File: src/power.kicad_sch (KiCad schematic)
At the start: 28 parts, among them U1 ECP5U_12_CABGA256, U12 TLV62569DRL, U13 TLV62569DRL, U14 TLV62569DRL

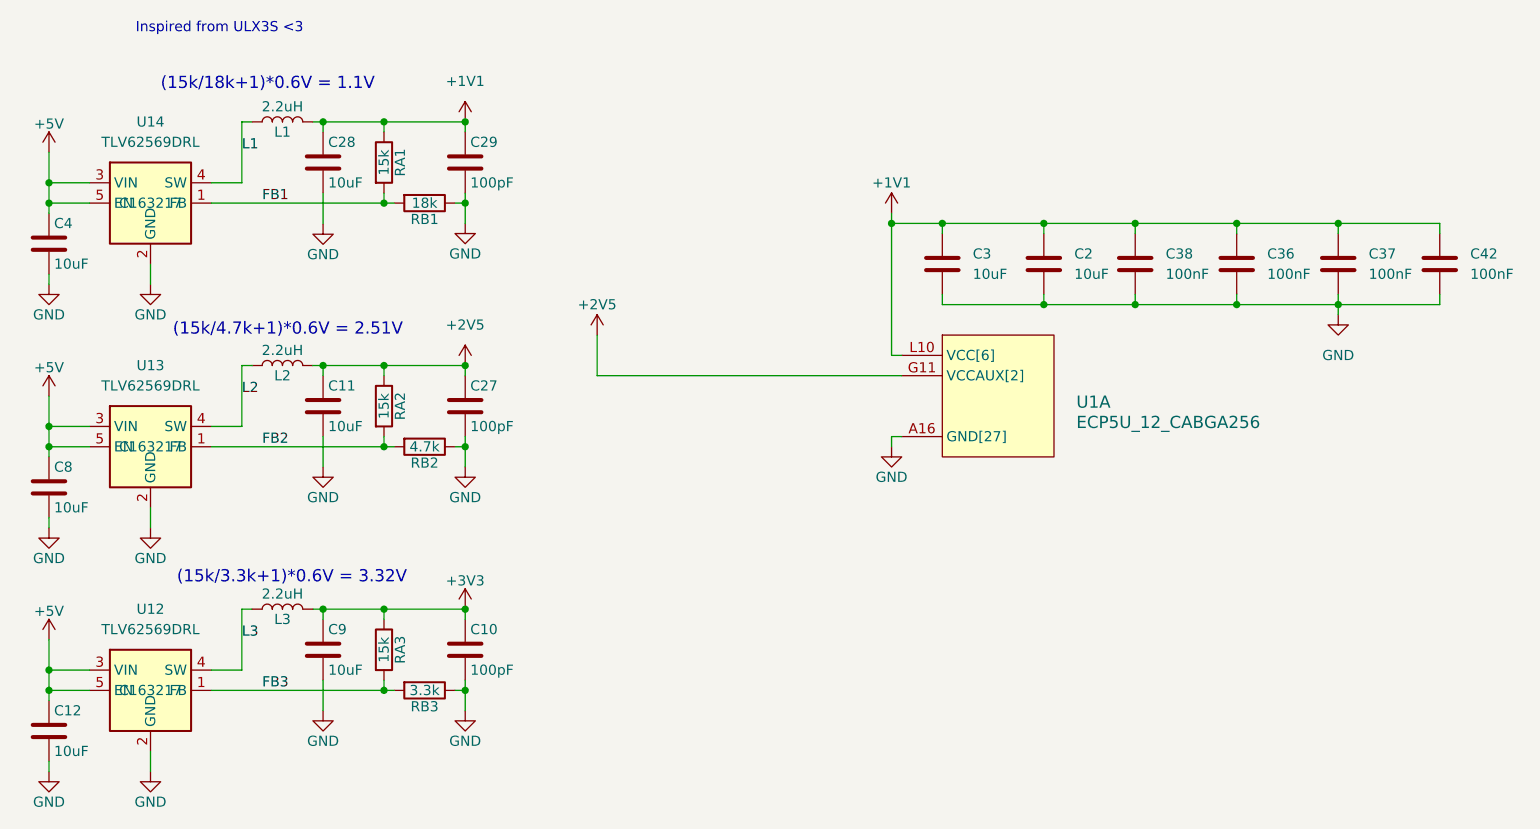
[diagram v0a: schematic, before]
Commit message: Rev 2
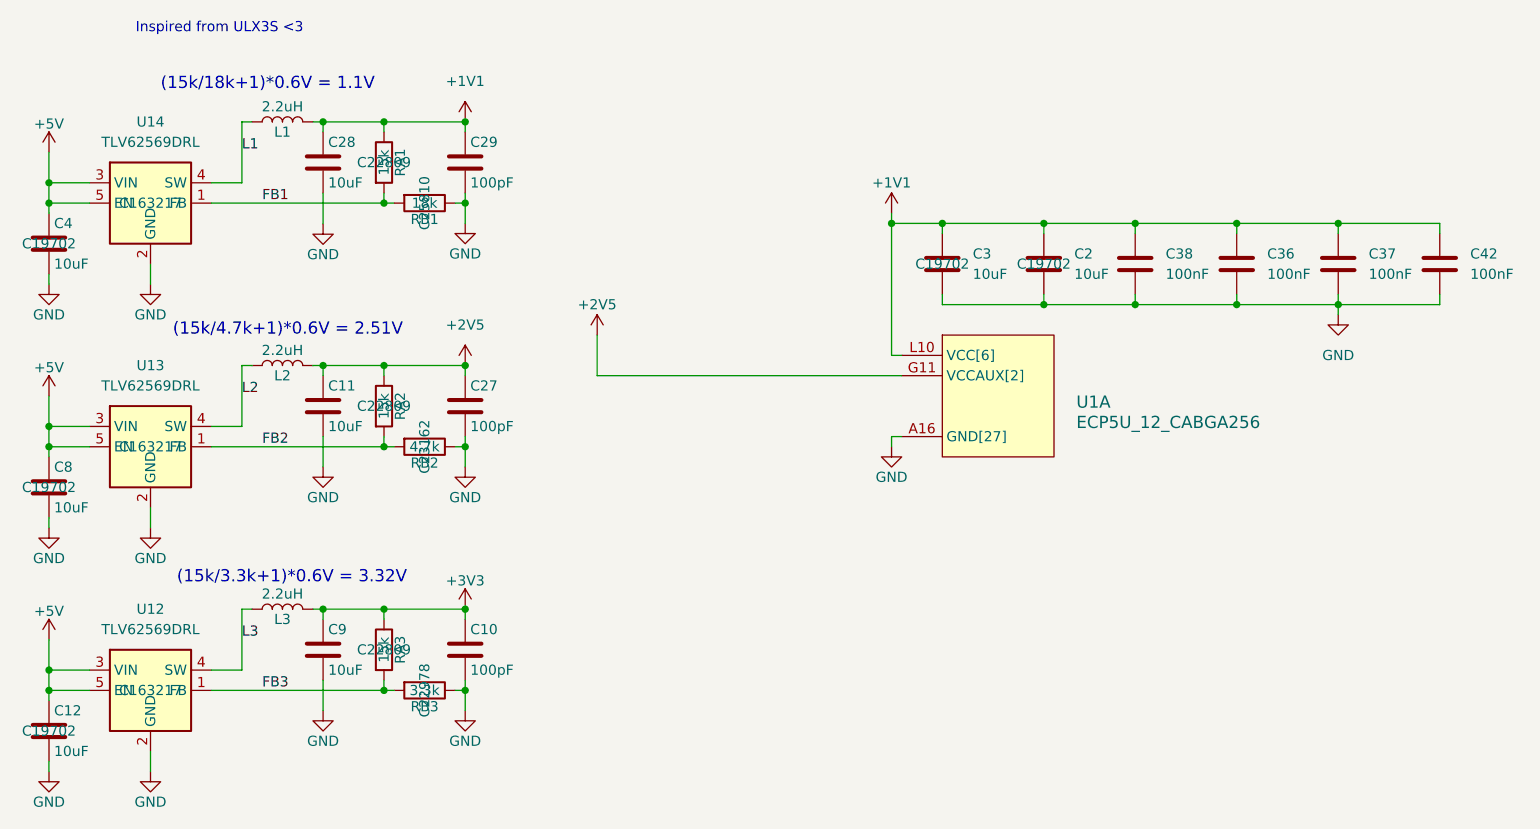
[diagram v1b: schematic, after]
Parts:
- C10, C27, C29: LCSC Part (none) -> C14858
- C11, C12, C2, C28, C3, C4, C8, C9: LCSC Part (none) -> C19702
- C36, C37, C38, C42: LCSC Part (none) -> C1525
- RA1, RA2, RA3: LCSC Part (none) -> C22809
- RB1: LCSC Part (none) -> C25810
- RB2: LCSC Part (none) -> C23162
- RB3: LCSC Part (none) -> C22978
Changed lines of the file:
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@@
 			)
 		)
+		(property "LCSC Part" "C19702"
+			(at 72.39 72.39 0)
+			(effects
+				(font
+					(size 1.27 1.27)
+				)
+			)
+		)
 		(pin "1"
 		)
@@
 			)
 		)
+		(property "LCSC Part" "C22809"
+			(at 114.3 62.23 0)
+			(effects
+				(font
+					(size 1.27 1.27)
+				)
+			)
+		)
 		(pin "1"
 		)
@@
 			)
 		)
+		(property "LCSC Part" "C25810"
+			(at 119.38 67.31 0)
+			(effects
+				(font
+					(size 1.27 1.27)
+				)
+			)
+		)
 		(pin "1"
 		)
@@
 			)
 		)
-		(property "LCSC Part" ""
+		(property "LCSC Part" "C19702"
 			(at 106.68 123.19 0)
 			(effects
@@
 			)
 		)
+		(property "LCSC Part" "C22809"
+			(at 114.3 123.19 0)
+			(effects
+				(font
+					(size 1.27 1.27)
+				)
+			)
+		)
 		(pin "1"
 		)
@@
 			)
 		)
+		(property "LCSC Part" "C22978"
+			(at 119.38 128.27 0)
+			(effects
+				(font
+					(size 1.27 1.27)
+				)
+			)
+		)
 		(pin "1"
 		)
@@
 			)
 		)
-		(property "LCSC Part" ""
+		(property "LCSC Part" "C14858"
 			(at 124.46 123.19 0)
 			(effects
@@
 			)
 		)
+		(property "LCSC Part" "C22809"
+			(at 114.3 92.71 0)
+			(effects
+				(font
+					(size 1.27 1.27)
+				)
+			)
+		)
 		(pin "1"
 		)
@@
 			)
 		)
+		(property "LCSC Part" "C23162"
+			(at 119.38 97.79 0)
+			(effects
+				(font
+					(size 1.27 1.27)
+				)
+			)
+		)
 		(pin "1"
 		)
@@
 			)
 		)
-		(property "LCSC Part" ""
+		(property "LCSC Part" "C1525"
 			(at 246.38 74.93 0)
 			(effects
@@
 			)
 		)
-		(property "LCSC Part" ""
+		(property "LCSC Part" "C14858"
 			(at 124.46 92.71 0)
 			(effects
@@
 			)
 		)
+		(property "LCSC Part" "C19702"
+			(at 72.39 133.35 0)
+			(effects
+				(font
+					(size 1.27 1.27)
+				)
+			)
+		)
 		(pin "1"
 		)
@@
 			)
 		)
-		(property "LCSC Part" ""
+		(property "LCSC Part" "C14858"
 			(at 124.46 62.23 0)
 			(effects
@@
 			)
 		)
-		(property "LCSC Part" ""
+		(property "LCSC Part" "C1525"
 			(at 208.28 74.93 0)
 			(effects
@@
 			)
 		)
+		(property "LCSC Part" "C19702"
+			(at 72.39 102.87 0)
+			(effects
+				(font
+					(size 1.27 1.27)
+				)
+			)
+		)
 		(pin "1"
 		)
@@
 			)
 		)
-		(property "LCSC Part" ""
+		(property "LCSC Part" "C1525"
 			(at 233.68 74.93 0)
 			(effects
@@
 			)
 		)
+		(property "LCSC Part" "C19702"
+			(at 196.85 74.93 0)
+			(effects
+				(font
+					(size 1.27 1.27)
+				)
+			)
+		)
 		(pin "2"
 		)
@@
 			)
 		)
-		(property "LCSC Part" ""
+		(property "LCSC Part" "C19702"
 			(at 106.68 92.71 0)
 			(effects
@@
 			)
 		)
-		(property "LCSC Part" ""
+		(property "LCSC Part" "C1525"
 			(at 220.98 74.93 0)
 			(effects
@@
 			)
 		)
+		(property "LCSC Part" "C19702"
+			(at 184.15 74.93 0)
+			(effects
+				(font
+					(size 1.27 1.27)
+				)
+			)
+		)
 		(pin "2"
 		)
@@
 			)
 		)
-		(property "LCSC Part" ""
+		(property "LCSC Part" "C19702"
 			(at 106.68 62.23 0)
 			(effects

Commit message: Tidy project
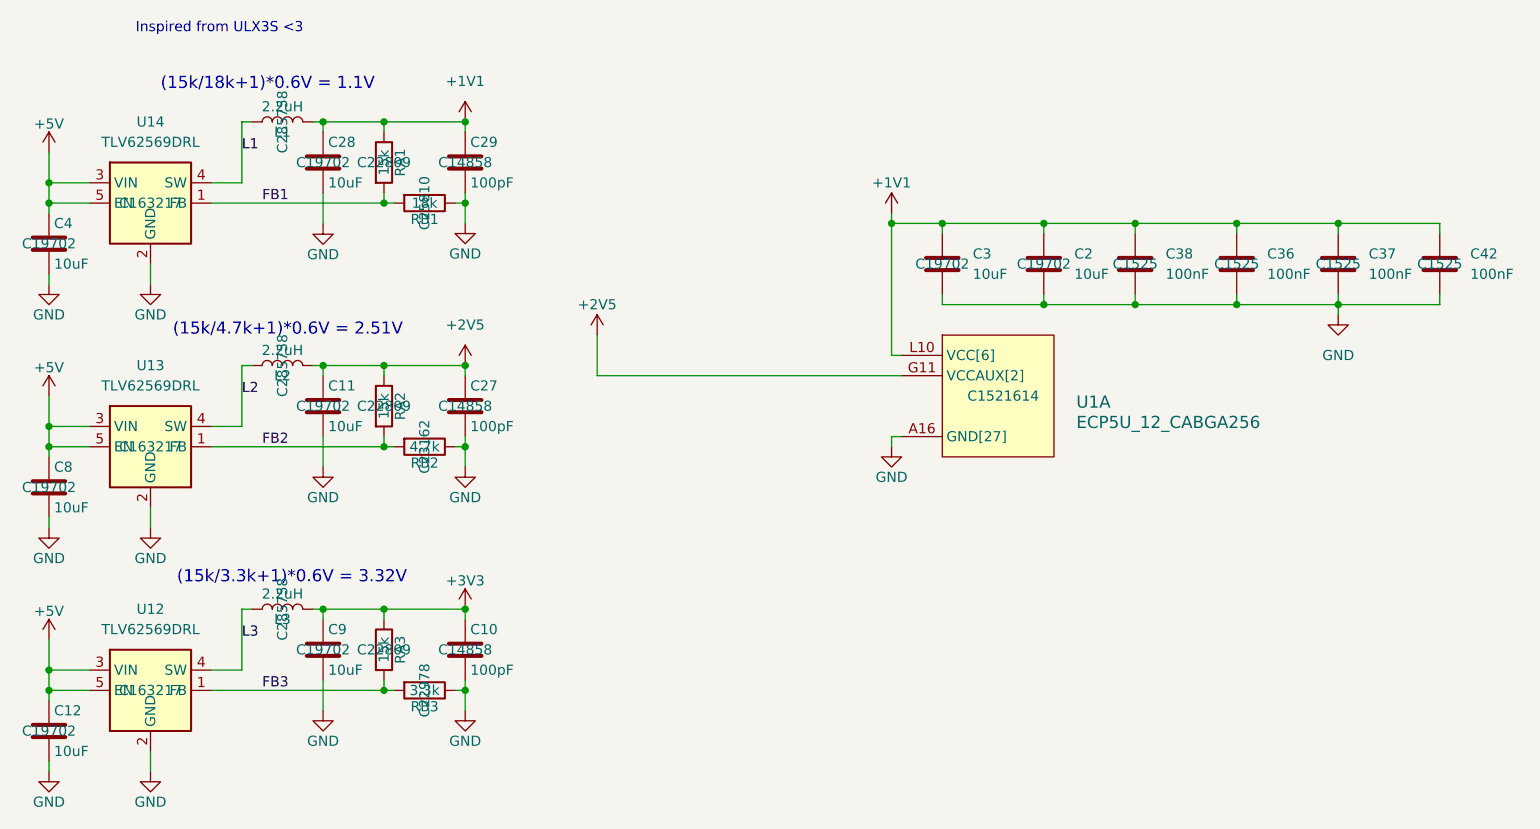
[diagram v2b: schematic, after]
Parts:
- C10, C27, C29: JLCPCB Part # (none) -> C14858; LCSC Part C14858 -> (none)
- C11, C12, C2, C28, C3, C4, C8, C9: JLCPCB Part # (none) -> C19702; LCSC Part C19702 -> (none)
- C36, C37, C38, C42: JLCPCB Part # (none) -> C1525; LCSC Part C1525 -> (none)
- L1, L2, L3: JLCPCB Part # (none) -> C285758; LCSC Part C285758 -> (none)
- RA1, RA2, RA3: JLCPCB Part # (none) -> C22809; LCSC Part C22809 -> (none)
- RB1: JLCPCB Part # (none) -> C25810; LCSC Part C25810 -> (none)
- RB2: JLCPCB Part # (none) -> C23162; LCSC Part C23162 -> (none)
- RB3: JLCPCB Part # (none) -> C22978; LCSC Part C22978 -> (none)
- U1: JLCPCB Part # (none) -> C1521614; LCSC Part C1521614 -> (none)
- U12, U13, U14: JLCPCB Part # (none) -> C163217; LCSC Part C163217 -> (none)
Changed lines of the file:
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@@
 			)
 		)
-		(property "LCSC Part" "C19702"
+		(property "JLCPCB Part #" "C19702"
 			(at 72.39 72.39 0)
 			(effects
@@
 			)
 		)
-		(property "LCSC Part" "C22809"
+		(property "JLCPCB Part #" "C22809"
 			(at 114.3 62.23 0)
 			(effects
@@
 			)
 		)
-		(property "LCSC Part" "C25810"
+		(property "JLCPCB Part #" "C25810"
 			(at 119.38 67.31 0)
 			(effects
@@
 			)
 		)
-		(property "LCSC Part" "C19702"
+		(property "JLCPCB Part #" "C19702"
 			(at 106.68 123.19 0)
 			(effects
@@
 					(size 1.27 1.27)
 				)
-				(hide yes)
 			)
 		)
@@
 			)
 		)
-		(property "LCSC Part" "C22809"
+		(property "JLCPCB Part #" "C22809"
 			(at 114.3 123.19 0)
 			(effects
@@
 			)
 		)
-		(property "LCSC Part" "C22978"
+		(property "JLCPCB Part #" "C22978"
 			(at 119.38 128.27 0)
 			(effects
@@
 			)
 		)
-		(property "LCSC Part" "C14858"
+		(property "JLCPCB Part #" "C14858"
 			(at 124.46 123.19 0)
 			(effects
@@
 					(size 1.27 1.27)
 				)
-				(hide yes)
 			)
 		)
@@
 			)
 		)
-		(property "LCSC Part" " C285758"
+		(property "JLCPCB Part #" " C285758"
 			(at 101.6 87.63 0)
 			(effects
@@
 					(size 1.27 1.27)
 				)
-				(hide yes)
 			)
 		)
@@
 			)
 		)
-		(property "LCSC Part" "C22809"
+		(property "JLCPCB Part #" "C22809"
 			(at 114.3 92.71 0)
 			(effects
@@
 			)
 		)
-		(property "LCSC Part" "C23162"
+		(property "JLCPCB Part #" "C23162"
 			(at 119.38 97.79 0)
 			(effects
@@
 			)
 		)
-		(property "LCSC Part" " C285758"
+		(property "JLCPCB Part #" " C285758"
 			(at 101.6 57.15 0)
 			(effects
@@
 					(size 1.27 1.27)
 				)
-				(hide yes)
 			)
 		)
@@
 			)
 		)
-		(property "LCSC Part" " C285758"
+		(property "JLCPCB Part #" " C285758"
 			(at 101.6 118.11 0)
 			(effects
@@
 					(size 1.27 1.27)
 				)
-				(hide yes)
 			)
 		)
@@
 			)
 		)
-		(property "LCSC Part" "C1525"
+		(property "JLCPCB Part #" "C1525"
 			(at 246.38 74.93 0)
 			(effects
@@
 					(size 1.27 1.27)
 				)
-				(hide yes)
 			)
 		)
@@
 			)
 		)
-		(property "LCSC Part" "C14858"
+		(property "JLCPCB Part #" "C14858"
 			(at 124.46 92.71 0)
 			(effects
@@
 					(size 1.27 1.27)
 				)
-				(hide yes)
 			)
 		)
@@
 			)
 		)
-		(property "LCSC Part" "C19702"
+		(property "JLCPCB Part #" "C19702"
 			(at 72.39 133.35 0)
 			(effects
@@
 			)
 		)
-		(property "LCSC Part" "C14858"
+		(property "JLCPCB Part #" "C14858"
 			(at 124.46 62.23 0)
 			(effects
@@
 					(size 1.27 1.27)
 				)
-				(hide yes)
 			)
 		)
@@
 			)
 		)
-		(property "LCSC Part" "C1525"
+		(property "JLCPCB Part #" "C1525"
 			(at 208.28 74.93 0)
 			(effects
@@
 					(size 1.27 1.27)
 				)
-				(hide yes)
 			)
 		)
@@
 			)
 		)
-		(property "LCSC Part" "C163217"
+		(property "JLCPCB Part #" "C163217"
 			(at 85.09 67.31 0)
 			(effects
@@
 			)
 		)
-		(property "LCSC Part" "C19702"
+		(property "JLCPCB Part #" "C19702"
 			(at 72.39 102.87 0)
 			(effects
@@
 			)
 		)
-		(property "LCSC Part" "C163217"
+		(property "JLCPCB Part #" "C163217"
 			(at 85.09 97.79 0)
 			(effects
@@
 			)
 		)
-		(property "LCSC Part" " C1521614"
+		(property "JLCPCB Part #" " C1521614"
 			(at 191.77 91.44 0)
 			(effects
@@
 					(size 1.27 1.27)
 				)
-				(hide yes)
 			)
 		)
@@
 			)
 		)
-		(property "LCSC Part" "C1525"
+		(property "JLCPCB Part #" "C1525"
 			(at 233.68 74.93 0)
 			(effects
@@
 					(size 1.27 1.27)
 				)
-				(hide yes)
 			)
 		)
@@
 			)
 		)
-		(property "LCSC Part" "C19702"
+		(property "JLCPCB Part #" "C19702"
 			(at 196.85 74.93 0)
 			(effects
@@
 			)
 		)
-		(property "LCSC Part" "C19702"
+		(property "JLCPCB Part #" "C19702"
 			(at 106.68 92.71 0)
 			(effects
@@
 					(size 1.27 1.27)
 				)
-				(hide yes)
 			)
 		)
@@
 			)
 		)
-		(property "LCSC Part" "C1525"
+		(property "JLCPCB Part #" "C1525"
 			(at 220.98 74.93 0)
 			(effects
@@
 					(size 1.27 1.27)
 				)
-				(hide yes)
 			)
 		)
@@
 			)
 		)
-		(property "LCSC Part" "C163217"
+		(property "JLCPCB Part #" "C163217"
 			(at 85.09 128.27 0)
 			(effects
@@
 			)
 		)
-		(property "LCSC Part" "C19702"
+		(property "JLCPCB Part #" "C19702"
 			(at 184.15 74.93 0)
 			(effects
@@
 			)
 		)
-		(property "LCSC Part" "C19702"
+		(property "JLCPCB Part #" "C19702"
 			(at 106.68 62.23 0)
 			(effects
@@
 					(size 1.27 1.27)
 				)
-				(hide yes)
 			)
 		)
